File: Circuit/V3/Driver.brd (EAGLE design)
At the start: 61 x 56 mm, 37 parts, among them IC1 DRV8303DCA

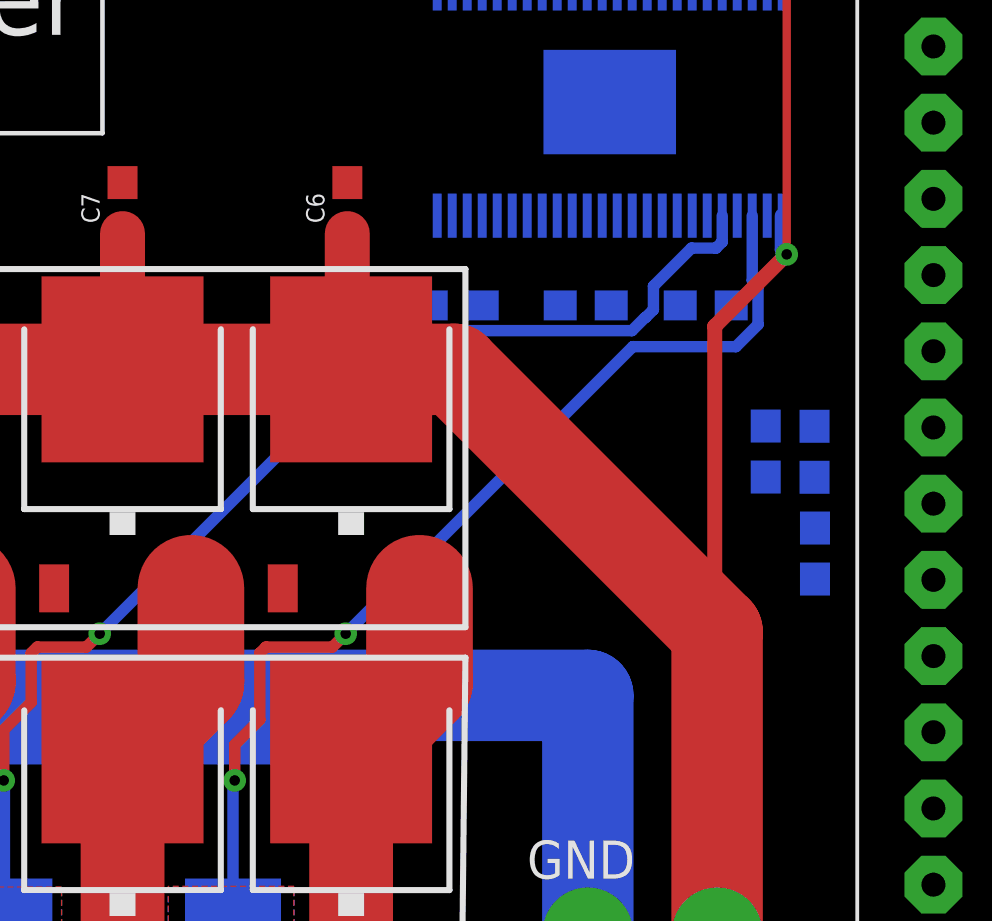
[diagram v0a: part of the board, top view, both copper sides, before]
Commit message: Fixed some bugs
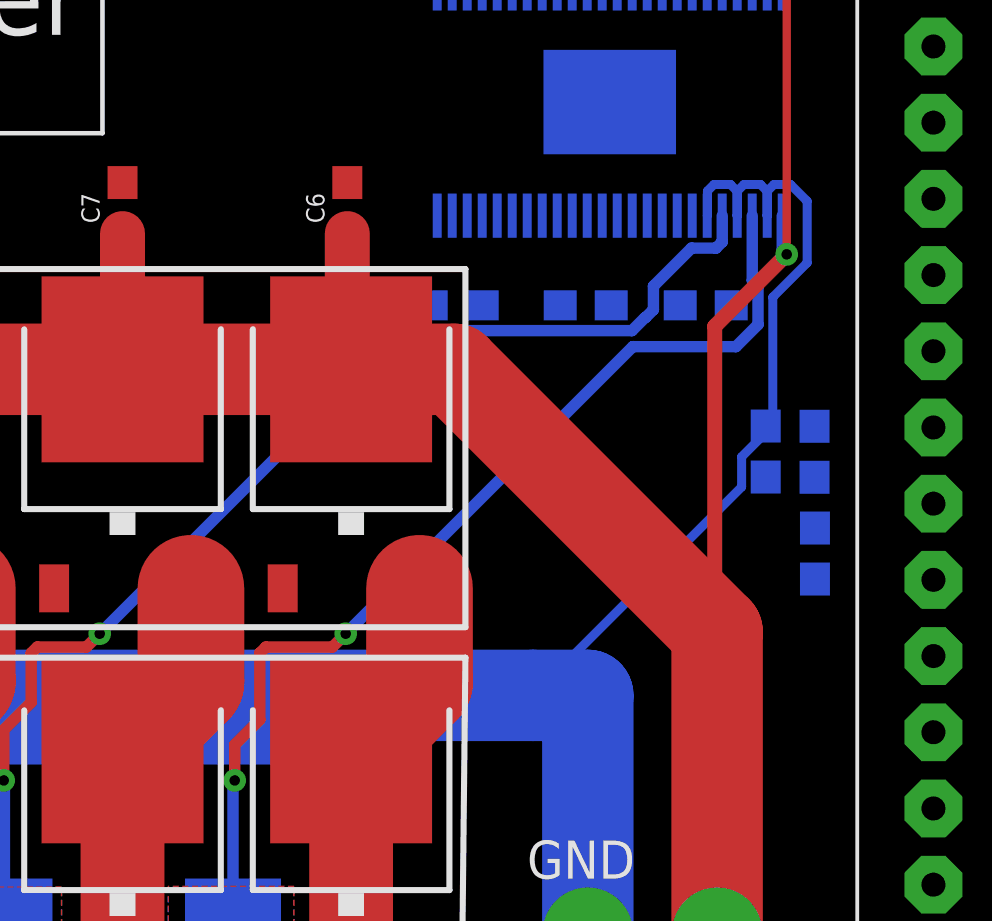
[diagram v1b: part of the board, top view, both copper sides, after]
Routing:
- net GND: track 38.5 -> 66.9 mm
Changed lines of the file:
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@@
 <contactref element="IC1" pad="30"/>
 <wire x1="29.07" y1="5.588" x2="29.07" y2="15" width="3.048" layer="16"/>
-<wire x1="29.07" y1="15" x2="17" y2="15" width="3.048" layer="16"/>
+<wire x1="29.07" y1="15" x2="27.25" y2="15" width="3.048" layer="16"/>
+<wire x1="27.25" y1="15" x2="17" y2="15" width="3.048" layer="16"/>
 <wire x1="17" y1="15" x2="9.5" y2="15" width="3.048" layer="16"/>
 <wire x1="8" y1="15" x2="9.5" y2="15" width="3.048" layer="16"/>
@@
 <contactref element="C16" pad="2"/>
 <contactref element="IC1" pad="3"/>
+<wire x1="34.82525625" y1="32.0289" x2="34.27474375" y2="32.0289" width="0.3" layer="16"/>
+<wire x1="35.05" y1="30.989" x2="35.0429" y2="30.9961" width="0.3" layer="16"/>
+<wire x1="34.0571" y1="30.9961" x2="34.05" y2="30.989" width="0.3" layer="16"/>
+<wire x1="35.0429" y1="30.9961" x2="35.0429" y2="31.81125625" width="0.3" layer="16"/>
+<wire x1="35.0429" y1="31.81125625" x2="34.82525625" y2="32.0289" width="0.3" layer="16"/>
+<wire x1="34.27474375" y1="32.0289" x2="34.0571" y2="31.81125625" width="0.3" layer="16"/>
+<wire x1="34.0571" y1="31.81125625" x2="34.0571" y2="30.9961" width="0.3" layer="16"/>
+<wire x1="33.82525625" y1="32.0289" x2="33.27474375" y2="32.0289" width="0.3" layer="16"/>
+<wire x1="34.05" y1="30.989" x2="34.0429" y2="30.9961" width="0.3" layer="16"/>
+<wire x1="33.0571" y1="30.9961" x2="33.05" y2="30.989" width="0.3" layer="16"/>
+<wire x1="34.0429" y1="30.9961" x2="34.0429" y2="31.81125625" width="0.3" layer="16"/>
+<wire x1="34.0429" y1="31.81125625" x2="33.82525625" y2="32.0289" width="0.3" layer="16"/>
+<wire x1="33.27474375" y1="32.0289" x2="33.0571" y2="31.81125625" width="0.3" layer="16"/>
+<wire x1="33.0571" y1="31.81125625" x2="33.0571" y2="30.9961" width="0.3" layer="16"/>
+<wire x1="35.27474375" y1="32.0289" x2="35.82525625" y2="32.0289" width="0.3" layer="16"/>
+<wire x1="34.1976" y1="22.95225625" x2="34.1976" y2="21.9476" width="0.3" layer="16"/>
+<wire x1="34.1976" y1="21.9476" x2="27.25" y2="15" width="0.3" layer="16"/>
+<wire x1="35.0576" y1="31.81175625" x2="35.27474375" y2="32.0289" width="0.3" layer="16"/>
+<wire x1="35.2358" y1="23.99045625" x2="34.1976" y2="22.95225625" width="0.3" layer="16"/>
+<wire x1="35.82525625" y1="32.0289" x2="36.3806" y2="31.47355625" width="0.3" layer="16"/>
+<wire x1="36.3806" y1="31.47355625" x2="36.3806" y2="29.41808125" width="0.3" layer="16"/>
+<wire x1="35.05" y1="30.989" x2="35.0576" y2="30.9966" width="0.3" layer="16"/>
+<wire x1="35.0576" y1="30.9966" x2="35.0576" y2="31.81175625" width="0.3" layer="16"/>
+<wire x1="35.2358" y1="28.27328125" x2="35.2358" y2="23.99045625" width="0.3" layer="16"/>
+<wire x1="36.3806" y1="29.41808125" x2="35.2358" y2="28.27328125" width="0.3" layer="16"/>
 <wire x1="37.1" y1="42.45" x2="55.831" y2="49.33" width="0" layer="19" extent="16-16"/>
 <wire x1="35.177" y1="42.9" x2="37.1" y2="42.45" width="0" layer="19" extent="1-16"/>
@@
 <wire x1="29.8" y1="34.777" x2="35.55" y2="38.565" width="0" layer="19" extent="16-16"/>
 <wire x1="33.05" y1="30.989" x2="29.8" y2="34.777" width="0" layer="19" extent="16-16"/>
-<wire x1="34.05" y1="30.989" x2="33.05" y2="30.989" width="0" layer="19" extent="16-16"/>
-<wire x1="35.05" y1="30.989" x2="34.05" y2="30.989" width="0" layer="19" extent="16-16"/>
+<wire x1="23.46" y1="5.868" x2="24.25" y2="5.5" width="0" layer="19" extent="1-1"/>
+<wire x1="5.94" y1="11.518" x2="8" y2="15" width="0" layer="19" extent="16-16"/>
+<wire x1="13.56" y1="11.518" x2="17.243" y2="13.595" width="0" layer="19" extent="16-16"/>
 <wire x1="25.05" y1="38.565" x2="29.8" y2="34.777" width="0" layer="19" extent="16-16"/>
 <wire x1="25.05" y1="30.989" x2="29.8" y2="34.777" width="0" layer="19" extent="16-16"/>
@@
 <wire x1="13.56" y1="32.092" x2="21.053" y2="32.092" width="0" layer="19" extent="1-1"/>
 <wire x1="5.94" y1="32.092" x2="13.56" y2="32.092" width="0" layer="19" extent="1-1"/>
-<wire x1="8" y1="15" x2="5.94" y2="32.092" width="0" layer="19" extent="1-16"/>
-<wire x1="23.46" y1="5.868" x2="24.25" y2="5.5" width="0" layer="19" extent="1-1"/>
-<wire x1="5.94" y1="11.518" x2="8" y2="15" width="0" layer="19" extent="16-16"/>
-<wire x1="13.56" y1="11.518" x2="17.243" y2="13.595" width="0" layer="19" extent="16-16"/>
 <wire x1="40.591" y1="6.15" x2="29.07" y2="5.588" width="0" layer="19" extent="1-1"/>
 <wire x1="40.591" y1="3.61" x2="40.591" y2="6.15" width="0" layer="19" extent="1-1"/>
@@
 <contactref element="C14" pad="1"/>
 <contactref element="C15" pad="1"/>
-<wire x1="35.55" y1="30.989" x2="35.55" y2="29.85" width="0.5" layer="16"/>
-<wire x1="35.55" y1="29.85" x2="35.7" y2="29.7" width="0.5" layer="16"/>
 <via x="35.7" y="29.7" extent="1-16" drill="0.35"/>
 <wire x1="35.7" y1="29.7" x2="33.3" y2="27.3" width="0.5" layer="1"/>
@@
 <wire x1="34.917803125" y1="41.682196875" x2="35.7" y2="40.9" width="0.28" layer="1"/>
 <wire x1="35.7" y1="40.9" x2="35.7" y2="29.7" width="0.28" layer="1"/>
+<wire x1="35.55" y1="30.989" x2="35.55" y2="29.85" width="0.38" layer="16"/>
+<wire x1="35.55" y1="29.85" x2="35.7" y2="29.7" width="0.38" layer="16"/>
 <wire x1="33.38" y1="5.588" x2="33.3" y2="5.1" width="0" layer="19" extent="1-1"/>
 </signal>
@@
 <contactref element="IC1" pad="12"/>
 <contactref element="D2" pad="A"/>
-<wire x1="55.831" y1="3.61" x2="29.55" y2="38.565" width="0" layer="19" extent="16-16"/>
+<wire x1="29.55" y1="38.565" x2="55.831" y2="3.61" width="0" layer="19" extent="16-16"/>
 <wire x1="33.423" y1="42.9" x2="29.55" y2="38.565" width="0" layer="19" extent="1-16"/>
 </signal>
@@
 <mfgpreviewcolor name="substratecolor" color="0xFF786E46"/>
 </mfgpreviewcolors>
-<errors>
-</errors>
 </board>
 </drawing>
